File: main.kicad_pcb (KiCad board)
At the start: 4 copper layers, 145.7 x 89.5 mm, 0 parts

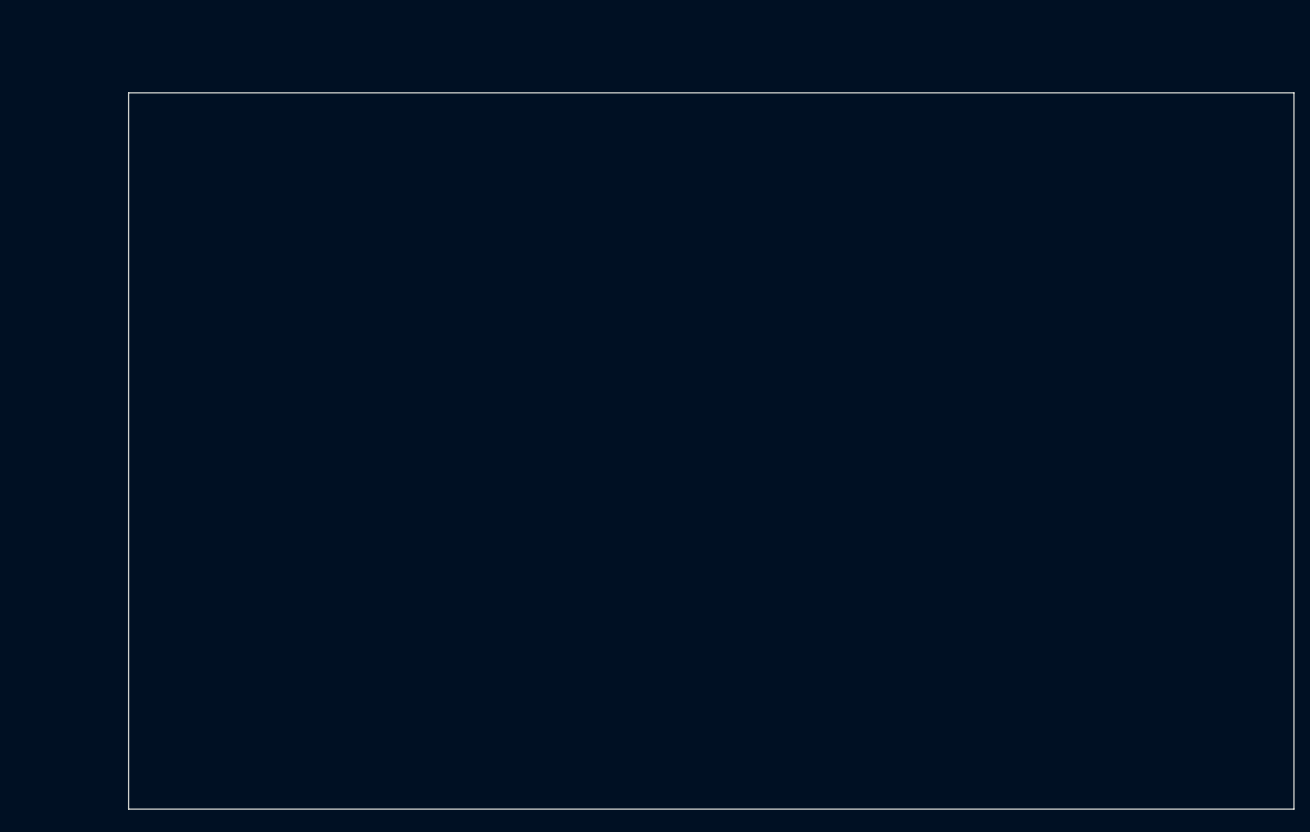
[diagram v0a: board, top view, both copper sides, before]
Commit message: update pcb
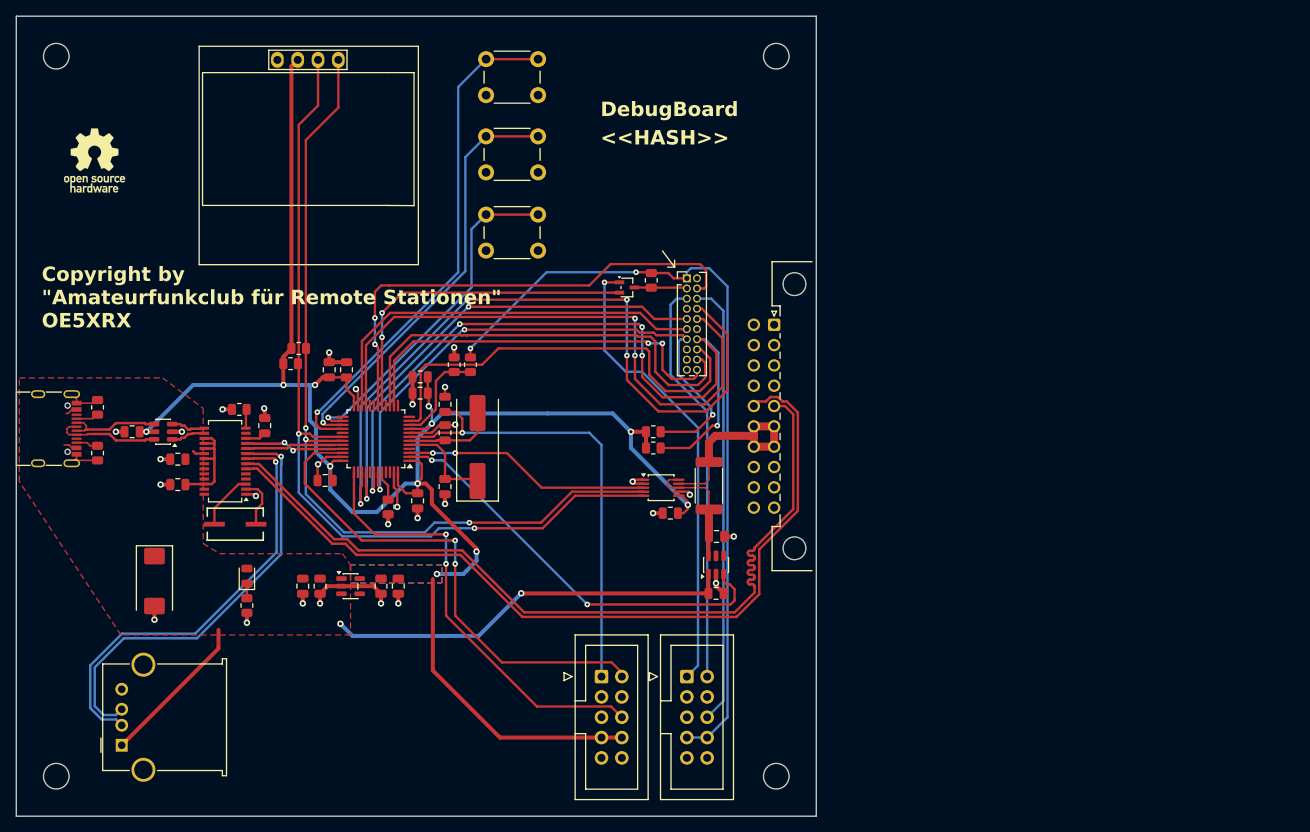
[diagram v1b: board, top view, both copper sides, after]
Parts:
- added #SYM101: OSHW-Logo_7.5x8mm_SilkScreen, Symbol:OSHW-Logo_7.5x8mm_SilkScreen, F.Cu at (85.3, 49.2)
- added Brd701: SSD1306, PRJ:128x64OLED, F.Cu at (111.8, 47.2)
- added C201: 100nF, Capacitor_SMD:C_0805_2012Metric, F.Cu at (129.1, 79.6)
- added C202: 30pF, Capacitor_SMD:C_0805_2012Metric, F.Cu at (129.1, 89.9)
- added C203: 100nF, Capacitor_SMD:C_0805_2012Metric, F.Cu at (125.7, 91.7)
- added C204: 30pF, Capacitor_SMD:C_0805_2012Metric, F.Cu at (129.1, 83.2)
- added C205: 100nF, Capacitor_SMD:C_0805_2012Metric, F.Cu at (114.6, 75.3)
- added C206: 100nF, Capacitor_SMD:C_0805_2012Metric, F.Cu at (114.1, 89.2)
- added C207: 4.7u/10V/X5R, Capacitor_SMD:C_0805_2012Metric, F.Cu at (116.8, 75.3)
- added C208: 100nF, Capacitor_SMD:C_0805_2012Metric, F.Cu at (126.0, 76.2)
- added C209: 4.7u/10V/X5R, Capacitor_SMD:C_0805_2012Metric, F.Cu at (126.0, 78.3)
- added C301: 100u / 25V, Capacitor_Tantalum_SMD:CP_EIA-7343-43_Kemet-X, F.Cu at (92.8, 101.7)
- added C302: 100nF, Capacitor_SMD:C_0805_2012Metric, F.Cu at (90.0, 83.1)
- added C401: 100nF, Capacitor_SMD:C_0805_2012Metric, F.Cu at (113.5, 102.4)
- added C402: 1uF, Capacitor_SMD:C_0805_2012Metric, F.Cu at (111.3, 102.4)
- added C403: 1uF, Capacitor_SMD:C_0805_2012Metric, F.Cu at (121.1, 102.4)
- added C404: 100nF, Capacitor_SMD:C_0805_2012Metric, F.Cu at (123.2, 102.4)
- added C501: 10uF, Capacitor_SMD:C_0805_2012Metric, F.Cu at (95.7, 89.7)
- added C502: 10uF, Capacitor_SMD:C_0805_2012Metric, F.Cu at (106.5, 82.3)
- added C503: 100nF, Capacitor_SMD:C_0805_2012Metric, F.Cu at (95.7, 86.5)
- added C801: 4.7u/10V/X5R, Capacitor_SMD:C_0805_2012Metric, F.Cu at (163.0, 103.3)
- added C802: 4.7u/10V/X5R, Capacitor_SMD:C_0805_2012Metric, F.Cu at (163.0, 96.2)
- added C901: 100n, Capacitor_SMD:C_0805_2012Metric, F.Cu at (157.2, 93.3)
- added D1001: BAT54CW, Package_TO_SOT_SMD:SOT-323_SC-70, F.Cu at (151.8, 65.0)
- added D301: LED, LED_SMD:LED_0805_2012Metric, F.Cu at (104.3, 101.1)
- added H101: MountingHole, MountingHole:MountingHole_3.2mm_M3, F.Cu at (80.5, 36.1)
- added H102: MountingHole, MountingHole:MountingHole_3.2mm_M3, F.Cu at (80.5, 126.1)
- added H103: MountingHole, MountingHole:MountingHole_3.2mm_M3, F.Cu at (170.5, 36.1)
- added H104: MountingHole, MountingHole:MountingHole_3.2mm_M3, F.Cu at (170.5, 126.1)
- added J1001: Conn_02x10_Odd_Even, Connector_PinHeader_1.27mm:PinHeader_2x10_P1.27mm_Vertical, F.Cu at (159.3, 63.9)
- added J1002: Conn_02x10_Row_Letter_First, PRJ:PCN10-20P-2.54DS, F.Cu at (170.2, 69.7)
- added J1101: Conn_02x05_Odd_Even, Connector_IDC:IDC-Header_2x05_P2.54mm_Vertical, F.Cu at (148.6, 113.7)
- added J1201: Conn_02x05_Odd_Even, Connector_IDC:IDC-Header_2x05_P2.54mm_Vertical, F.Cu at (159.3, 113.7)
- added J301: USB_C_Receptacle_USB2.0_16P, Connector_USB:USB_C_Receptacle_G-Switch_GT-USB-7010ASV, F.Cu at (79.3, 82.7)
- added J601: USB_A, Connector_USB:USB_A_Molex_67643_Horizontal, F.Cu at (88.7, 122.3)
- added R1001: 10k, Resistor_SMD:R_0805_2012Metric, F.Cu at (154.9, 64.2)
- added R201: 2k2, Resistor_SMD:R_0805_2012Metric, F.Cu at (122.0, 92.5)
- added R202: 4k7, Resistor_SMD:R_0805_2012Metric, F.Cu at (155.1, 85.1)
- added R203: 4k7, Resistor_SMD:R_0805_2012Metric, F.Cu at (155.1, 83.1)
- added R204: 4k7, Resistor_SMD:R_0805_2012Metric, F.Cu at (109.8, 74.6)
- added R205: 4k7, Resistor_SMD:R_0805_2012Metric, F.Cu at (110.8, 72.7)
- added R206: 100k, Resistor_SMD:R_0805_2012Metric, F.Cu at (130.2, 74.7)
- added R207: 100k, Resistor_SMD:R_0805_2012Metric, F.Cu at (132.3, 74.7)
- added R301: 5k1, Resistor_SMD:R_0805_2012Metric, F.Cu at (85.7, 80.0)
- added R302: 5k1, Resistor_SMD:R_0805_2012Metric, F.Cu at (85.7, 85.7)
- added R303: 1k, Resistor_SMD:R_0805_2012Metric, F.Cu at (104.3, 104.8)
- added R501: 2k7, Resistor_SMD:R_0805_2012Metric, F.Cu at (103.4, 80.3)
- added R901: 10m, Resistor_SMD:R_2512_6332Metric, F.Cu at (162.1, 89.8)
- added SW701: SW_Push, Button_Switch_THT:SW_PUSH_6mm, F.Cu at (134.2, 36.5)
- added SW702: SW_Push, Button_Switch_THT:SW_PUSH_6mm, F.Cu at (134.2, 46.2)
- added SW703: SW_Push, Button_Switch_THT:SW_PUSH_6mm, F.Cu at (134.2, 55.9)
- added U201: STM32F302CBTx, Package_QFP:LQFP-48_7x7mm_P0.5mm, F.Cu at (120.5, 84.0)
- added U301: USBLC6-2SC6, Package_TO_SOT_SMD:SOT-23-6, F.Cu at (93.8, 83.1)
- added U401: TLV73333PQDBVRQ1, Package_TO_SOT_SMD:SOT-23-5, F.Cu at (117.3, 102.4)
- added U501: FE1.1s, Package_SO:SSOP-28_3.9x9.9mm_P0.635mm, F.Cu at (101.6, 86.8)
- added U801: TPS22917DBV, Package_TO_SOT_SMD:SOT-23-6, F.Cu at (163.0, 99.7)
- added U901: INA226, Package_SO:VSSOP-10_3x3mm_P0.5mm, F.Cu at (156.1, 90.1)
- added Y201: 8MHz / 20pF, Crystal:Crystal_SMD_HC49-SD, F.Cu at (133.2, 85.0)
- added Y501: 12MHz, PRJ:M49S-SMD, F.Cu at (102.9, 94.6)
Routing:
- net +3V3: track 0.00 -> 238.0 mm, vias 0 -> 11
- net /Debug-Controller/I2C_SCL: track 0.00 -> 108.2 mm, vias 0 -> 2
- net /Debug-Controller/I2C_SDA: track 0.00 -> 106.9 mm, vias 0 -> 3
- net /DUT Interface Header/USB-: track 0.00 -> 104.5 mm
- net /DUT Interface Header/USB+: track 0.00 -> 104.4 mm
- net /DUT Interface Header/VCC_3V3: track 0.00 -> 99.4 mm, vias 0 -> 2
- net /DUT Interface Header/I2C_SCK: track 0.00 -> 95.8 mm, vias 0 -> 5
- net /DUT Interface Header/UART0_RX: track 0.00 -> 92.5 mm, vias 0 -> 4
- net +5V: track 0.00 -> 75.5 mm, vias 0 -> 2
- net GND: track 0.00 -> 74.8 mm, vias 0 -> 29
- net /DUT Interface Header/I2C_SDA: track 0.00 -> 74.5 mm, vias 0 -> 3
- net /DUT Interface Header/UART1_RX: track 0.00 -> 73.7 mm, vias 0 -> 2
- net /Debug-Controller/BUTTON_UP: track 0.00 -> 64.6 mm, vias 0 -> 1
- net /Debug-Controller/SWDIO: track 0.00 -> 63.3 mm, vias 0 -> 2
- net /DUT Interface Header/BOOT0: track 0.00 -> 60.8 mm, vias 0 -> 2
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- added copper zone on B.Cu, net +3V3
- added copper zone on F.Cu, net +3V3
- added copper zone on F.Cu, net +5V
- added copper zone on In1.Cu, net GND
- added copper zone on In2.Cu, net GND
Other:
- board size 145.7 x 89.5 mm -> 100 x 100 mm
- board text added: "<<HASH>>"
- board text added: "Copyright by {dblquote}Amateurfunkclub für Remote Stationen{dblquote} OE5XRX"
- board text added: "DebugBoard"
